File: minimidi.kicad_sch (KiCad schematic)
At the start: 75 parts, among them J1 ST7735R, SW1 SW_Push, SW10 SW_Push, SW11 SW_Push, SW12 SW_Push, SW13 SW_Push, SW14 SW_Push, SW15 SW_Push, SW16 SW_Push, SW17 SW_Push, SW18 SW_Push, SW19 SW_Push, SW2 SW_Push, SW20 SW_Push, SW21 SW_Push, SW22 SW_Push, SW23 SW_Push, SW24 SW_Push, SW25 RotaryEncoder_Switch_MP, SW26 RotaryEncoder_Switch_MP, SW27 SW_Push, SW28 SW_Push, SW29 SW_Push, SW3 SW_Push, SW30 SW_Push, SW31 SW_Push, SW32 SW_Push, SW33 SW_Push, SW34 SW_Push, SW35 RESET, SW36 SW_Push, SW37 SW_Push, SW4 SW_Push, SW5 SW_Push, SW6 SW_Push, SW7 SW_Push, SW8 SW_Push, SW9 SW_Push

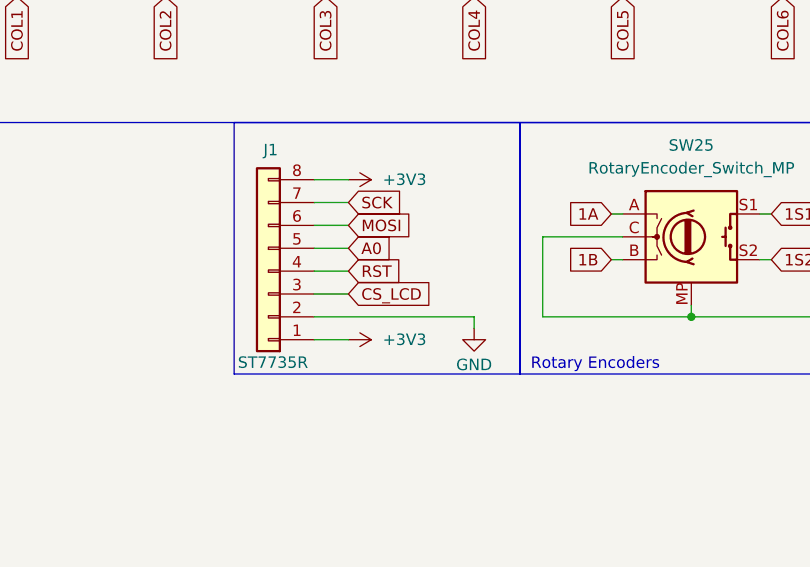
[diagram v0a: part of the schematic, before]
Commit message: Making PCBs
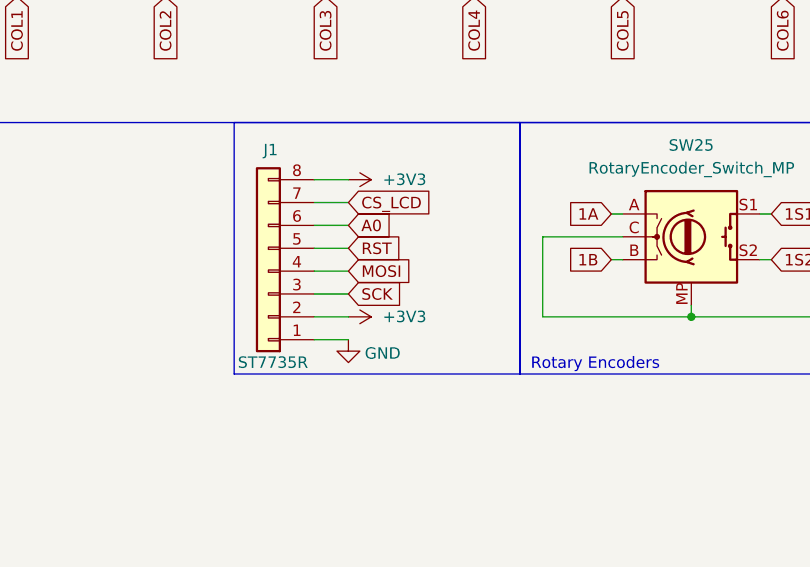
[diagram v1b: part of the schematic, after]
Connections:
- net +3V3: now also J1.2 (Pin_2); no longer J1.1 (Pin_1)
- net A0: now also J1.6 (Pin_6); no longer J1.5 (Pin_5)
- net CS_LCD: now also J1.7 (Pin_7); no longer J1.3 (Pin_3)
- net GND: now also J1.1 (Pin_1); no longer J1.2 (Pin_2)
- net MOSI: now also J1.4 (Pin_4); no longer J1.6 (Pin_6)
- net RST: now also J1.5 (Pin_5); no longer J1.4 (Pin_4)
- net SCK: now also J1.3 (Pin_3); no longer J1.7 (Pin_7)
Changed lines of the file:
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@@
 	(wire
 		(pts
-			(xy 182.88 146.05) (xy 186.69 146.05)
-		)
-		(stroke
-			(width 0)
-			(type default)
-		)
-	)
-	(wire
-		(pts
 			(xy 246.38 24.13) (xy 246.38 44.45)
 		)
@@
 	(wire
 		(pts
-			(xy 182.88 153.67) (xy 186.69 153.67)
-		)
-		(stroke
-			(width 0)
-			(type default)
-		)
-	)
-	(wire
-		(pts
 			(xy 215.9 100.33) (xy 215.9 104.14)
 		)
@@
 	(wire
 		(pts
-			(xy 182.88 148.59) (xy 186.69 148.59)
-		)
-		(stroke
-			(width 0)
-			(type default)
-		)
-	)
-	(wire
-		(pts
 			(xy 261.62 63.5) (xy 259.08 63.5)
 		)
@@
 	(wire
 		(pts
+			(xy 182.88 151.13) (xy 186.69 151.13)
+		)
+		(stroke
+			(width 0)
+			(type default)
+		)
+	)
+	(wire
+		(pts
 			(xy 251.46 104.14) (xy 251.46 87.63)
 		)
@@
 	(wire
 		(pts
+			(xy 182.88 146.05) (xy 186.69 146.05)
+		)
+		(stroke
+			(width 0)
+			(type default)
+		)
+	)
+	(wire
+		(pts
 			(xy 113.03 165.1) (xy 113.03 170.18)
 		)
@@
 	(wire
 		(pts
+			(xy 182.88 156.21) (xy 186.69 156.21)
+		)
+		(stroke
+			(width 0)
+			(type default)
+		)
+	)
+	(wire
+		(pts
 			(xy 184.15 104.14) (xy 191.77 104.14)
 		)
@@
 	(wire
 		(pts
+			(xy 182.88 161.29) (xy 186.69 161.29)
+		)
+		(stroke
+			(width 0)
+			(type default)
+		)
+	)
+	(wire
+		(pts
 			(xy 154.94 91.44) (xy 154.94 100.33)
 		)
@@
 	(wire
 		(pts
-			(xy 182.88 161.29) (xy 186.69 161.29)
+			(xy 132.08 195.58) (xy 132.08 190.5)
 		)
 		(stroke
@@
 	(wire
 		(pts
-			(xy 132.08 195.58) (xy 132.08 190.5)
+			(xy 217.17 123.19) (xy 217.17 104.14)
 		)
 		(stroke
@@
 	(wire
 		(pts
-			(xy 217.17 123.19) (xy 217.17 104.14)
+			(xy 246.38 24.13) (xy 248.92 24.13)
 		)
 		(stroke
@@
 	(wire
 		(pts
-			(xy 246.38 24.13) (xy 248.92 24.13)
+			(xy 200.66 82.55) (xy 200.66 57.15)
 		)
 		(stroke
@@
 	(wire
 		(pts
-			(xy 200.66 82.55) (xy 200.66 57.15)
+			(xy 219.71 57.15) (xy 219.71 39.37)
 		)
 		(stroke
@@
 	(wire
 		(pts
-			(xy 219.71 57.15) (xy 219.71 39.37)
+			(xy 251.46 104.14) (xy 259.08 104.14)
 		)
 		(stroke
@@
 	(wire
 		(pts
-			(xy 251.46 104.14) (xy 259.08 104.14)
+			(xy 182.88 148.59) (xy 186.69 148.59)
 		)
 		(stroke
@@
 	(wire
 		(pts
+			(xy 182.88 153.67) (xy 186.69 153.67)
+		)
+		(stroke
+			(width 0)
+			(type default)
+		)
+	)
+	(wire
+		(pts
 			(xy 154.94 91.44) (xy 171.45 91.44)
 		)
@@
 	(wire
 		(pts
-			(xy 182.88 151.13) (xy 186.69 151.13)
-		)
-		(stroke
-			(width 0)
-			(type default)
-		)
-	)
-	(wire
-		(pts
 			(xy 234.95 104.14) (xy 242.57 104.14)
 		)
@@
 	(wire
 		(pts
-			(xy 200.66 158.75) (xy 200.66 160.02)
-		)
-		(stroke
-			(width 0)
-			(type default)
-		)
-	)
-	(wire
-		(pts
 			(xy 41.91 187.96) (xy 41.91 195.58)
 		)
@@
 	(wire
 		(pts
+			(xy 182.88 158.75) (xy 186.69 158.75)
+		)
+		(stroke
+			(width 0)
+			(type default)
+		)
+	)
+	(wire
+		(pts
 			(xy 248.92 71.12) (xy 266.7 71.12)
 		)
@@
 	(wire
 		(pts
-			(xy 182.88 158.75) (xy 200.66 158.75)
-		)
-		(stroke
-			(width 0)
-			(type default)
-		)
-	)
-	(wire
-		(pts
 			(xy 171.45 44.45) (xy 171.45 53.34)
 		)
@@
 	(wire
 		(pts
-			(xy 182.88 156.21) (xy 186.69 156.21)
-		)
-		(stroke
-			(width 0)
-			(type default)
-		)
-	)
-	(wire
-		(pts
 			(xy 200.66 123.19) (xy 200.66 104.14)
 		)
@@
 	(global_label "SCK"
 		(shape input)
-		(at 186.69 146.05 0)
+		(at 186.69 156.21 0)
 		(fields_autoplaced yes)
 		(effects
@@
 		)
 		(property "Intersheetrefs" "${INTERSHEET_REFS}"
-			(at 193.4247 146.05 0)
+			(at 193.4247 156.21 0)
 			(effects
 				(font
@@
 	(global_label "CS_LCD"
 		(shape input)
-		(at 186.69 156.21 0)
+		(at 186.69 146.05 0)
 		(fields_autoplaced yes)
 		(effects
@@
 		)
 		(property "Intersheetrefs" "${INTERSHEET_REFS}"
-			(at 196.6904 156.21 0)
+			(at 196.6904 146.05 0)
 			(effects
 				(font
@@
 	(global_label "RST"
 		(shape input)
-		(at 186.69 153.67 0)
+		(at 186.69 151.13 0)
 		(fields_autoplaced yes)
 		(effects
@@
 		)
 		(property "Intersheetrefs" "${INTERSHEET_REFS}"
-			(at 193.1223 153.67 0)
+			(at 193.1223 151.13 0)
 			(effects
 				(font
@@
 	(global_label "A0"
 		(shape input)
-		(at 186.69 151.13 0)
+		(at 186.69 148.59 0)
 		(fields_autoplaced yes)
 		(effects
@@
 		)
 		(property "Intersheetrefs" "${INTERSHEET_REFS}"
-			(at 191.9733 151.13 0)
+			(at 191.9733 148.59 0)
 			(effects
 				(font
@@
 	(global_label "MOSI"
 		(shape input)
-		(at 186.69 148.59 0)
+		(at 186.69 153.67 0)
 		(fields_autoplaced yes)
 		(effects
@@
 		)
 		(property "Intersheetrefs" "${INTERSHEET_REFS}"
-			(at 194.2714 148.59 0)
+			(at 194.2714 153.67 0)
 			(effects
 				(font
@@
 	(symbol
 		(lib_id "power:+3V3")
-		(at 186.69 161.29 270)
+		(at 186.69 158.75 270)
 		(unit 1)
 		(exclude_from_sim no)
@@
 		(fields_autoplaced yes)
 		(property "Reference" "#PWR05"
-			(at 182.88 161.29 0)
+			(at 182.88 158.75 0)
 			(effects
 				(font
@@
 		)
 		(property "Value" "+3V3"
-			(at 190.5 161.2899 90)
+			(at 190.5 158.7499 90)
 			(effects
 				(font
@@
 		)
 		(property "Footprint" ""
-			(at 186.69 161.29 0)
+			(at 186.69 158.75 0)
 			(effects
 				(font
@@
 		)
 		(property "Datasheet" ""
-			(at 186.69 161.29 0)
+			(at 186.69 158.75 0)
 			(effects
 				(font
@@
 		)
 		(property "Description" "Power symbol creates a global label with name \"+3V3\""
-			(at 186.69 161.29 0)
+			(at 186.69 158.75 0)
 			(effects
 				(font
@@
 	(symbol
 		(lib_id "power:GND")
-		(at 200.66 160.02 0)
+		(at 186.69 161.29 0)
 		(unit 1)
 		(exclude_from_sim no)
@@
 		(dnp no)
 		(property "Reference" "#PWR06"
-			(at 200.66 166.37 0)
+			(at 186.69 167.64 0)
 			(effects
 				(font
@@
 		)
 		(property "Value" "GND"
-			(at 200.66 164.084 0)
+			(at 190.5 162.814 0)
 			(effects
 				(font
@@
 		)
 		(property "Footprint" ""
-			(at 200.66 160.02 0)
+			(at 186.69 161.29 0)
 			(effects
 				(font
@@
 		)
 		(property "Datasheet" ""
-			(at 200.66 160.02 0)
+			(at 186.69 161.29 0)
 			(effects
 				(font
@@
 		)
 		(property "Description" "Power symbol creates a global label with name \"GND\" , ground"
-			(at 200.66 160.02 0)
+			(at 186.69 161.29 0)
 			(effects
 				(font
